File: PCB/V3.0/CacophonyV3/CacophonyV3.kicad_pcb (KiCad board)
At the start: 2 copper layers, 61.1 x 47 mm, 28 parts, among them J1 Conn_01x04, J2 Conn_01x05, J3 Conn_01x03, J4 Conn_01x03, J5 Conn_01x03, J6 Conn_01x02

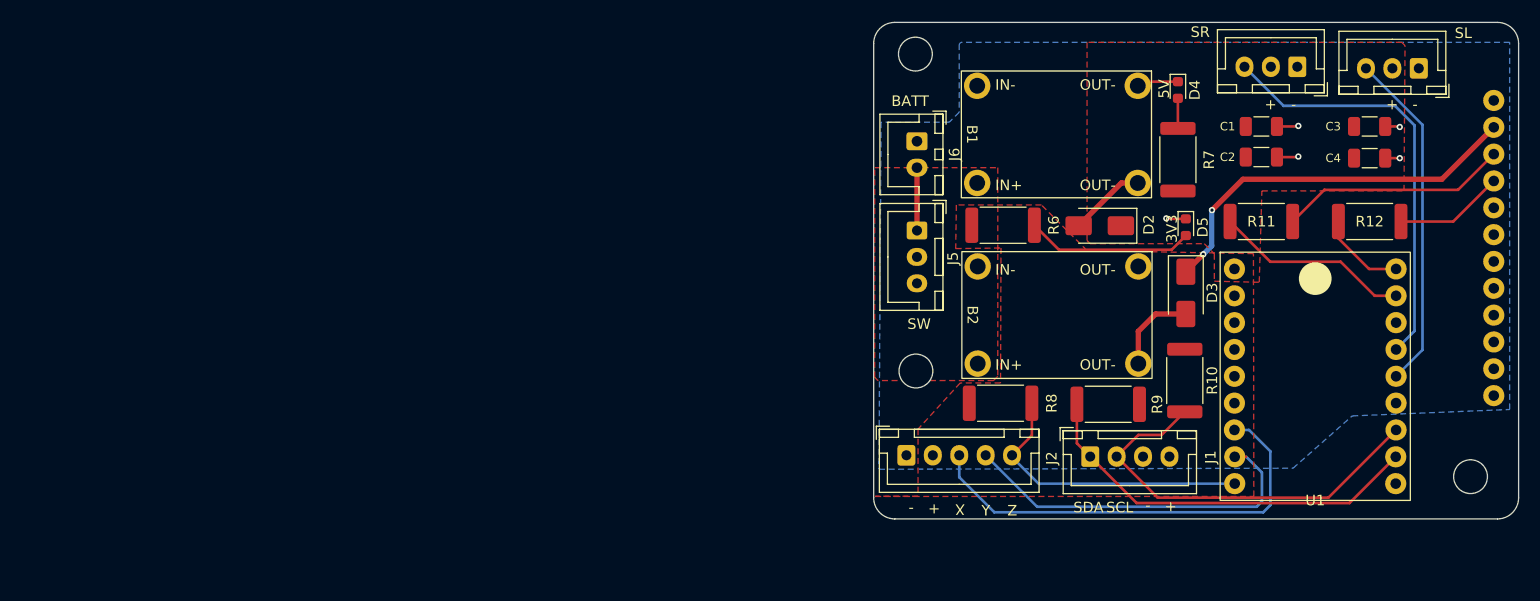
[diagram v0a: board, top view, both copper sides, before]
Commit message: New PCB
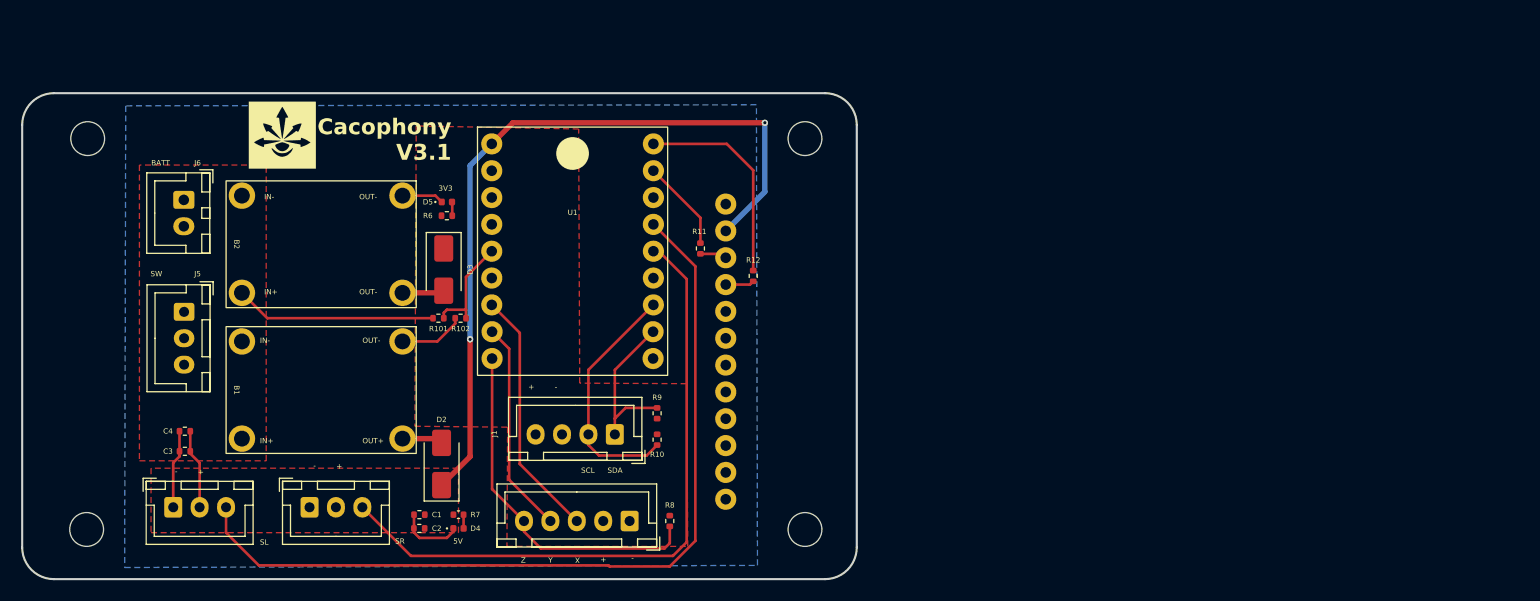
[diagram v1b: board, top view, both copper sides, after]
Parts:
- added R101: 200k, Resistor_SMD:R_0402_1005Metric, F.Cu at (75.3, 80.0)
- added R102: 100k, Resistor_SMD:R_0402_1005Metric, F.Cu at (77.4, 80.0)
- added REF**: MountingHole_3.2mm_M3, MountingHole:MountingHole_3.2mm_M3, F.Cu at (42.1, 63.0)
- C1, C2, C3, C4: footprint Capacitor_SMD:C_1206_3216Metric -> Resistor_SMD:R_0402_1005Metric
- D4, D5: footprint LED_SMD:LED_0603_1608Metric -> LED_SMD:LED_0402_1005Metric
- R10, R11, R12, R6, R8, R9: footprint Resistor_SMD:R_2512_6332Metric -> Resistor_SMD:R_0402_1005Metric
- R7: footprint Resistor_SMD:R_2512_6332Metric -> Capacitor_SMD:C_0402_1005Metric
- moved REF** 131.1 mm to (42.0, 100.0)
- moved J4 125.0 mm to (50.2, 97.9), turned to 0 degrees
- moved C3 116.3 mm to (51.3, 92.6), turned to 180 degrees
- moved C4 115.1 mm to (51.3, 90.7), turned to 180 degrees
- moved J3 102.4 mm to (63.1, 97.9), turned to 0 degrees
- moved C1 87.8 mm to (73.5, 98.6), turned to 180 degrees
- moved C2 87.1 mm to (73.5, 99.9), turned to 180 degrees
- moved D4 79.7 mm to (77.2, 99.9), turned to 0 degrees
- moved R7 75.9 mm to (77.2, 98.6), turned to 0 degrees
- moved B1 73.7 mm to (55.7, 86.8)
- moved IC1 73.4 mm to (103.5, 67.7)
- moved U1 71.3 mm to (88.0, 85.4)
- moved D3 70.3 mm to (75.8, 75.4)
- moved D5 70.0 mm to (76.1, 69.0), turned to 0 degrees
- moved B2 70.0 mm to (55.7, 73.0)
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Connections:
- IC1 pad 2: +3.3V -> +5V
- U1 pad 13: /PWM_R -> /PWM_L
- U1 pad 14: /PWM_L -> /PWM_R
- U1 pad 5: unconnected-(U1-IO2-Pad5) -> /VOut
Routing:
- net +5V: track 0.00 -> 80.3 mm, vias 0 -> 2
- net /PWM_L: track 32.4 -> 80.8 mm
- net +3.3V: track 36.8 -> 0.00 mm, vias 2 -> 0
- net /SDA: track 38.0 -> 15.6 mm
- net /PWM_R: track 40.3 -> 62.3 mm
- net Net-(IC1-TX): track 21.7 -> 2.55 mm
- net +9V: track 0.00 -> 19.1 mm
- net /JOYX: track 42.5 -> 23.8 mm
- net /SCL: track 38.9 -> 23.1 mm
- net Net-(D5-A): track 15.9 -> 1.31 mm
- net /JOYY: track 34.3 -> 20.2 mm
- net /ESP_Tx: track 8.25 -> 20.0 mm
- net GND: track 12.7 -> 23.8 mm, vias 5 -> 0
- net /VOut: track 0.00 -> 10.1 mm
- net /ESP_Rx: track 18.6 -> 8.69 mm
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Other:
- board size 61.1 x 47 mm -> 79 x 46 mm
- board text added: "OUT+"
